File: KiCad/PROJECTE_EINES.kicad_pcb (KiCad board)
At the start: 2 copper layers, 117.7 x 80.6 mm, 61 parts, among them J1 DE9_Pins_MountingHoles, J2 DE9_Pins_MountingHoles, J3 Conn_01x08_Pin, SW1 SW_DPDT_x2, SW2 SW_DPDT_x2, SW3 SW_DPDT_x2, U1 PIC24HJ128GP504-I_PT, U2 SN65HVD230, U3 VNH5019A-E, U4 LM2596S-5, U5 VNH5019A-E, U6 LM1117DT-3.3, Y1 8MHz

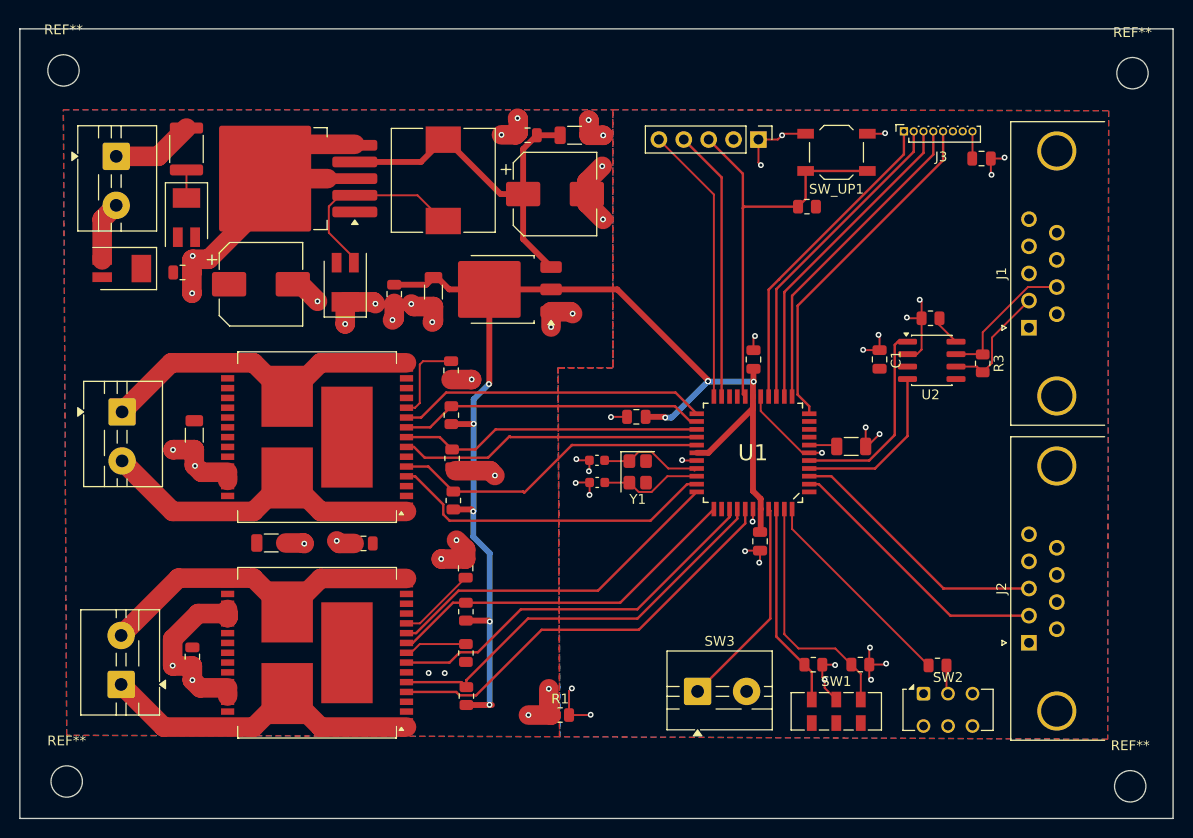
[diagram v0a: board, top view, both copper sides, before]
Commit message: Routing V3
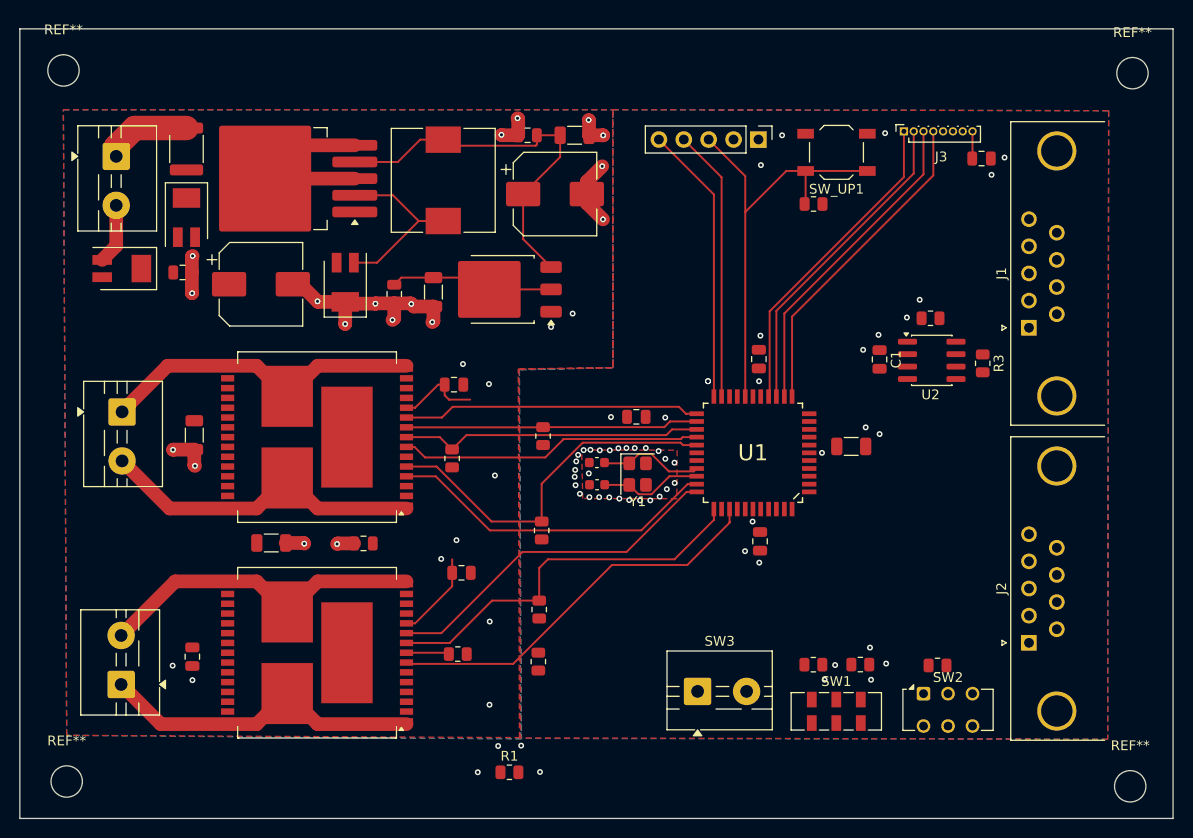
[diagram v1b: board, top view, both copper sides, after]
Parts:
- moved R_WIN_DIAGB1 9.60 mm to (137.1, 65.0)
- moved R_WIN_DIAGA1 9.52 mm to (137.0, 74.6)
- moved R_DIAGA_DOOR1 8.14 mm to (136.6, 88.0)
- moved R1 7.80 mm to (133.7, 99.3)
- moved R_DIAGB_DOOR1 7.48 mm to (136.7, 82.7)
- moved C_WIN_CP1 1.47 mm to (128.0, 59.7), turned to 180 degrees
- moved R_CS_DOOR1 0.83 mm to (128.4, 87.2), turned to 0 degrees
- moved R_MCLR1 0.72 mm to (164.7, 41.3)
- moved C_CP_DOOR1 0.62 mm to (128.8, 78.9), turned to 180 degrees
- moved C_AVDD1 0.55 mm to (159.1, 57.1)
- moved C_OSC2 0.23 mm to (142.6, 69.9)
- moved C_OSC1 0.23 mm to (142.6, 67.7)
- moved Y1 0.23 mm to (146.8, 68.8)
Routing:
- net +3.3V: track 131.2 -> 16.8 mm, vias 9 -> 7
- net GND: track 67.4 -> 0.00 mm, vias 29 -> 52
- net GNDPWR: track 116.7 -> 71.5 mm, vias 30 -> 28
- net DOOR_INA: track 43.4 -> 0.00 mm
- net DOOR_DIAGA: track 42.5 -> 0.00 mm
- net RFID_SCK: track 35.5 -> 0.00 mm
- net UART_RX: track 28.0 -> 0.00 mm
- net UART_TX: track 27.2 -> 0.00 mm
- net WIN_BTN_DOWN: track 24.9 -> 0.00 mm
- net WIN_LIMIT: track 21.7 -> 0.00 mm
- net DOOR_LOCK/UNLOCK: track 21.7 -> 0.00 mm
- net WIN_BTN_UP: track 20.9 -> 0.00 mm
- net CAN_TX: track 20.4 -> 0.00 mm
- net CAN_RX: track 17.2 -> 0.00 mm
- net /COMUNICACIONS/CANH: track 14.5 -> 0.00 mm
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- added copper zone on F.Cu, net GND

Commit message: Versió preliminar Routing Final
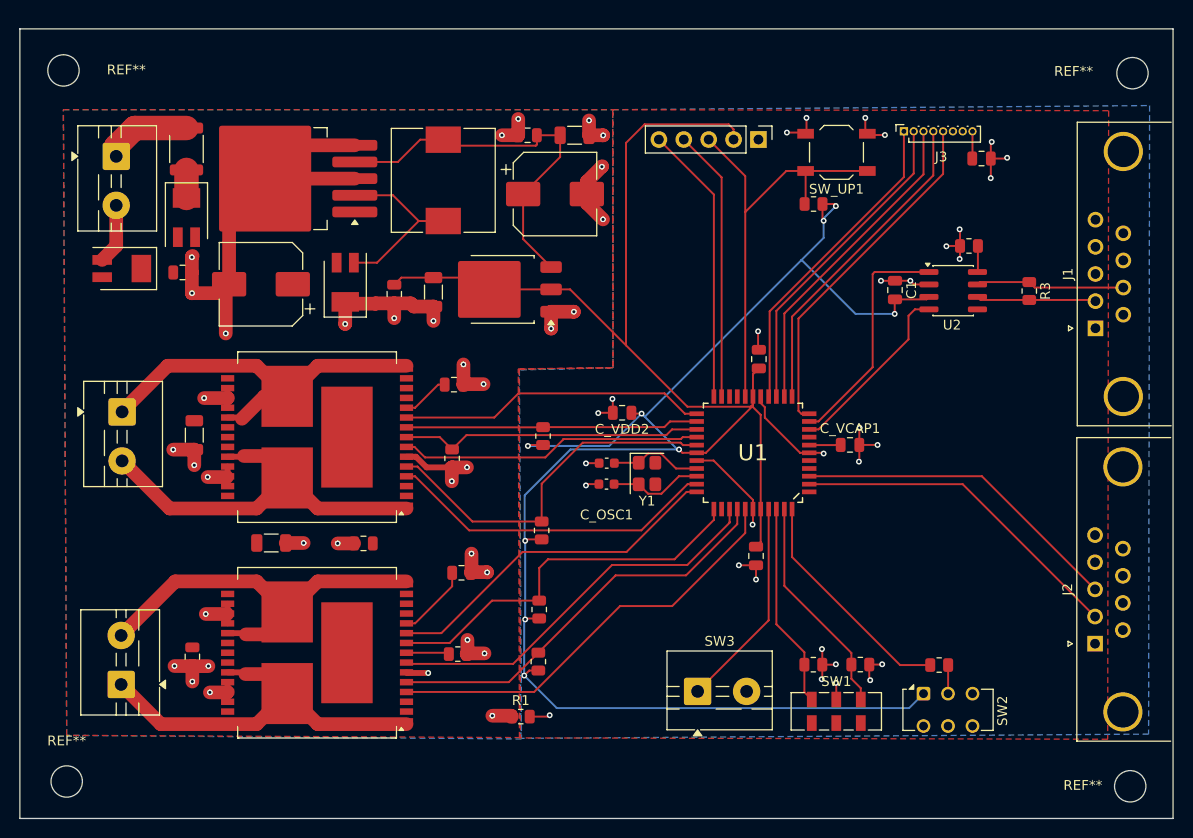
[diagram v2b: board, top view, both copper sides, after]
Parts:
- removed C_VDD1: 100nF, Capacitor_SMD:C_0805_2012Metric
- added C_VDD2: 100nF, Capacitor_SMD:C_0805_2012Metric, F.Cu at (145.2, 62.6)
- C_VCAP1: footprint Capacitor_SMD:C_1206_3216Metric -> Capacitor_SMD:C_0805_2012Metric
- moved R3 8.78 mm to (186.7, 50.2)
- moved R2 8.36 mm to (180.6, 45.6)
- moved U2 7.44 mm to (179.0, 50.1)
- moved C1 7.25 mm to (173.0, 50.1)
- moved J1 6.78 mm to (193.5, 54.0)
- moved J2 6.74 mm to (193.4, 86.2)
- moved R1 5.80 mm to (134.8, 93.6)
- moved C_BULK1 1.55 mm to (158.8, 77.2)
- moved C_OSC1 1.01 mm to (143.6, 67.7)
- moved C_OSC2 0.96 mm to (143.6, 69.9)
- moved Y1 0.96 mm to (147.7, 68.8)
- moved C_VCAP1 0.20 mm to (168.4, 65.9)
- moved R_Lock/Unlock1 0.17 mm to (177.5, 88.3)
- turned C_INBUCK2 to 180 degrees
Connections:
- net Net-(U1-OSC1/CLKI/CN30/RA2) renamed OSC_+
- net Net-(U1-OSC2/CLKO/CN29/RA3) renamed OSC_-
- U1 pad 10: unconnected-(U1-AN12/RP12(1)/CN14/PMD0/RB12-Pad10) -> CAN_TX
- U1 pad 4: CAN_RX -> unconnected-(U1-RP24(1)/CN20/PMA5/RC8-Pad4)
- U1 pad 5: CAN_TX -> unconnected-(U1-RP25(1)/CN19/PMA6/RC9-Pad5)
- U1 pad 9: unconnected-(U1-PGEC2/RP11(1)/CN15/PMD1/RB11-Pad9) -> CAN_RX
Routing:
- net +3.3V: track 16.8 -> 259.8 mm, vias 7 -> 9
- net GND: track 0.00 -> 69.3 mm, vias 52 -> 31
- net GNDPWR: track 71.5 -> 139.0 mm, vias 28 -> 35
- net DOOR_INA: track 0.00 -> 43.7 mm
- net DOOR_DIAGA: track 0.00 -> 42.0 mm
- net RFID_SCK: track 0.00 -> 35.9 mm
- net UART_RX: track 0.00 -> 34.8 mm
- net UART_TX: track 0.00 -> 33.9 mm
- net CAN_TX: track 0.00 -> 24.1 mm
- net DOOR_LOCK/UNLOCK: track 0.00 -> 23.6 mm
- net WIN_BTN_DOWN: track 0.00 -> 22.7 mm
- net WIN_LIMIT: track 0.00 -> 21.6 mm
- net WIN_BTN_UP: track 0.00 -> 20.9 mm
- net CAN_RX: track 0.00 -> 18.7 mm
- net /COMUNICACIONS/CANH: track 0.00 -> 15.2 mm
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- removed copper zone on F.Cu, net GND
